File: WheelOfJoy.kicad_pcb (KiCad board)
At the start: 2 copper layers, 89.2 x 87.9 mm, 39 parts, among them CN1 JOY1, CN2 JOY2, CN3 JOY3, CN4 JOY4, CN5 JOY5, CN6 JOY6, CN7 JOY7, CN8 JOY8, CN9 DB15F, U1 CD4051B, U2 CD4051B, U3 CD4051B, U4 CD4051B, U5 CD4051B

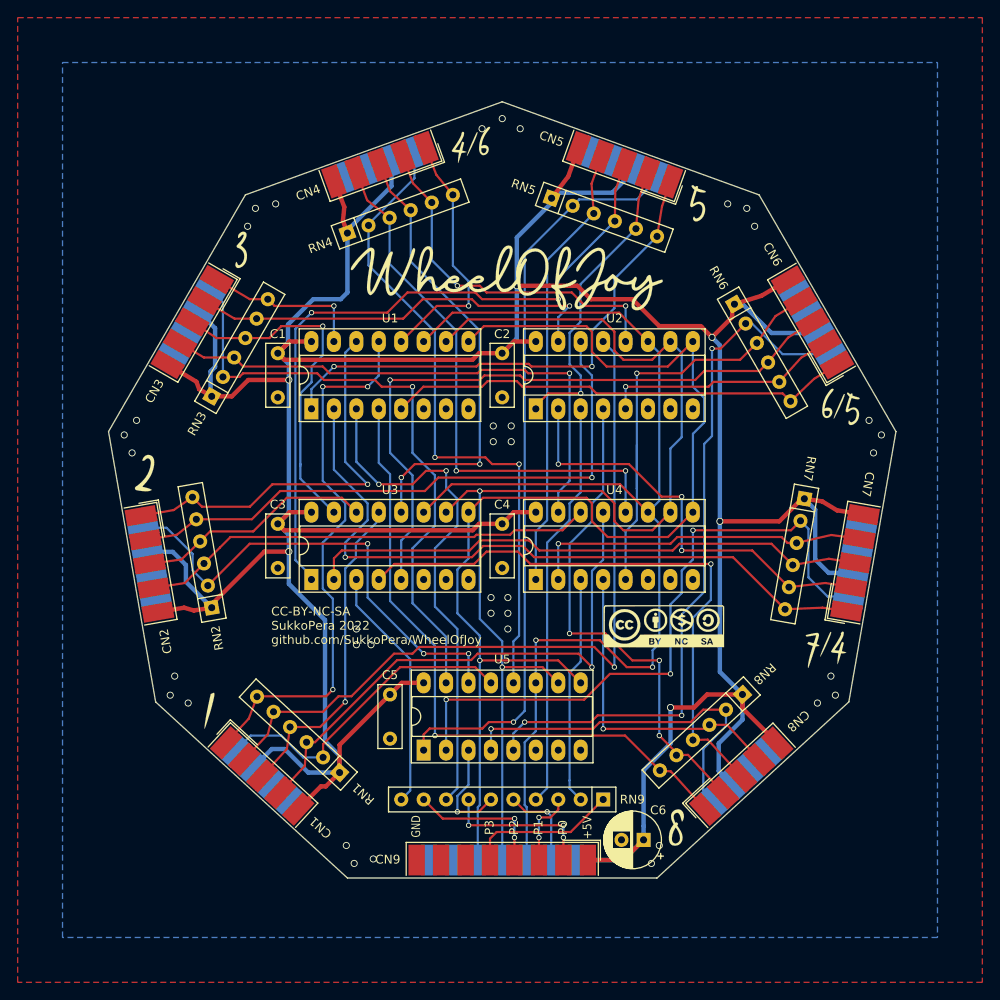
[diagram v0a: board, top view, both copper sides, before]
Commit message: WIP
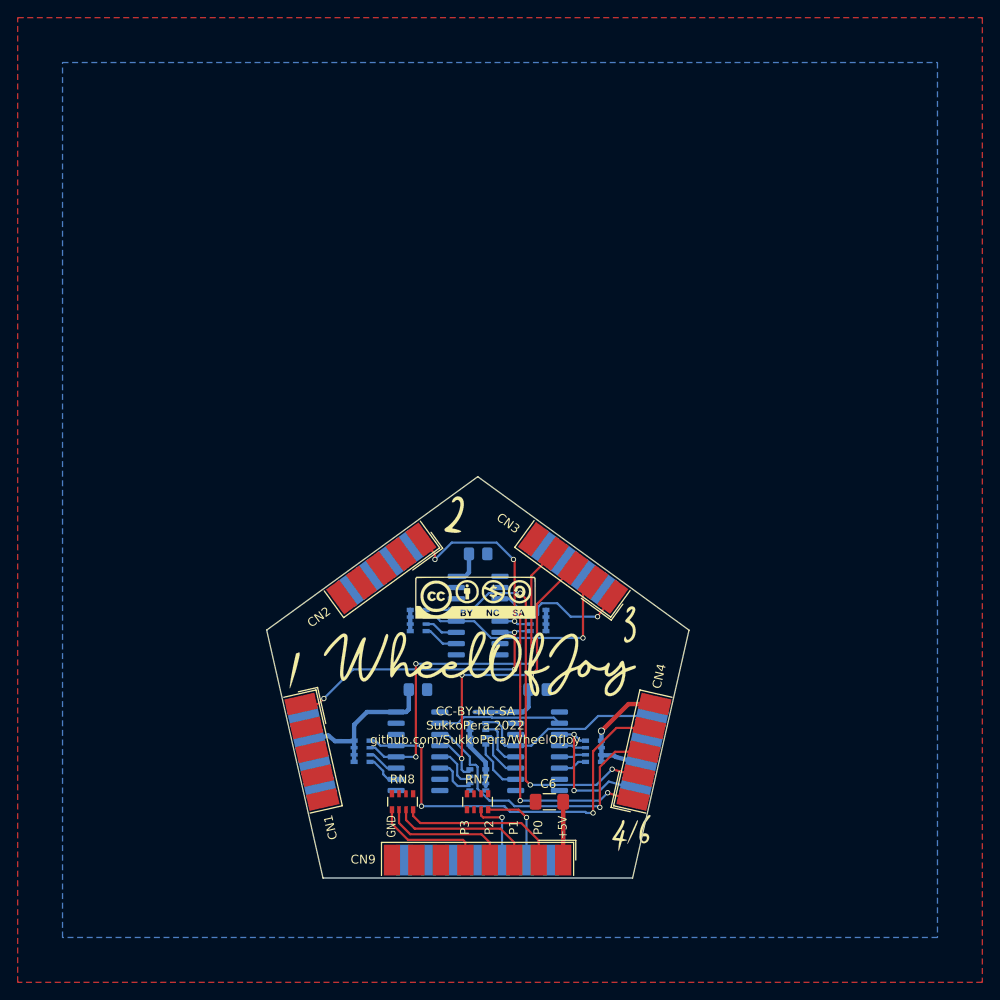
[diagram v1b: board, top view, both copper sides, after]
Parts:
- removed C4, C5: 100n, Capacitor_THT:C_Disc_D7.0mm_W2.5mm_P5.00mm
- removed CN5: JOY5, Connector_Dsub:DSUB-9_Male_EdgeMount_P2.77mm
- removed CN6: JOY6, Connector_Dsub:DSUB-9_Male_EdgeMount_P2.77mm
- removed CN7: JOY7, Connector_Dsub:DSUB-9_Male_EdgeMount_P2.77mm
- removed CN8: JOY8, Connector_Dsub:DSUB-9_Male_EdgeMount_P2.77mm
- removed RN9: 100, Resistor_THT:R_Array_SIP10
- removed U4, U5: CD4051B, Package_DIP:DIP-16_W7.62mm_Socket_LongPads
- removed V6: PORT5_NO, WheelOfJoy:port5
- removed V7: PORT6_NO, WheelOfJoy:port6
- removed V8: PORT7_NO, WheelOfJoy:port7
- removed V9: PORT8_NO, WheelOfJoy:port8
- C1, C2, C3: footprint Capacitor_THT:C_Disc_D7.0mm_W2.5mm_P5.00mm -> Capacitor_SMD:C_0805_2012Metric_Pad1.18x1.45mm_HandSolder; moved to B.Cu
- C6: footprint Capacitor_THT:CP_Radial_D6.3mm_P2.50mm -> Capacitor_SMD:C_1206_3216Metric_Pad1.33x1.80mm_HandSolder
- RN1, RN2, RN3, RN4, RN5, RN6: footprint Resistor_THT:R_Array_SIP6 -> Resistor_SMD:R_Array_Convex_4x0603; moved to B.Cu
- RN7, RN8: value 4.7k -> 100; footprint Resistor_THT:R_Array_SIP6 -> Resistor_SMD:R_Array_Convex_4x0603
- U1, U2, U3: value CD4051B -> 74LS153; footprint Package_DIP:DIP-16_W7.62mm_Socket_LongPads -> Package_SO:SOIC-16_3.9x9.9mm_P1.27mm; moved to B.Cu
- moved V5 80.0 mm to (166.0, 130.4)
- moved CN4 72.9 mm to (167.4, 121.2), turned to 77.2 degrees
- moved RN4 63.6 mm to (148.6, 124.4), turned to 180 degrees
- moved RN5 61.2 mm to (148.6, 119.2), turned to 180 degrees
- moved V4 61.1 mm to (166.8, 106.8)
- moved RN6 53.1 mm to (161.7, 121.2), turned to 180 degrees
- moved CN3 51.3 mm to (159.4, 100.4), turned to 144 degrees
- moved RN7 50.5 mm to (148.6, 126.9), turned to 90 degrees
- moved V0 43.8 mm to (148.8, 111.3)
- moved RN3 43.6 mm to (135.5, 121.2), turned to 180 degrees
- moved U2 41.0 mm to (141.8, 121.2), turned to 180 degrees
- moved RN8 40.4 mm to (140.1, 126.9), turned to 90 degrees
- moved C2 39.3 mm to (141.8, 114.2), turned to 0 degrees
- moved RN2 37.0 mm to (155.4, 106.4), turned to 180 degrees
- moved V3 35.4 mm to (146.4, 94.4)
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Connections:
- CN1 pad 9: (no net) -> Net-(CN1-Pad9)
- CN2 pad 9: (no net) -> Net-(CN2-Pad9)
- CN3 pad 9: (no net) -> Net-(CN3-Pad9)
- CN4 pad 9: (no net) -> Net-(CN4-Pad9)
- CN9 pad 11: /d5 -> Net-(CN9-Pad11)
- CN9 pad 14: (no net) -> Net-(CN9-Pad14)
- CN9 pad 6: (no net) -> /~reset
- CN9 pad 7: (no net) -> Net-(CN9-Pad7)
- RN1 pad 1: +5V -> Net-(CN4-Pad2)
- RN1 pad 2: Net-(CN1-Pad6) -> Net-(CN3-Pad2)
- RN1 pad 3: Net-(CN1-Pad4) -> Net-(CN2-Pad2)
- RN1 pad 4: Net-(CN1-Pad3) -> Net-(CN1-Pad2)
- RN1 pad 5: Net-(CN1-Pad2) -> +5V
- RN1 pad 6: Net-(CN1-Pad1) -> +5V
- RN2 pad 2: Net-(CN2-Pad6) -> +5V
- RN2 pad 3: Net-(CN2-Pad4) -> +5V
- RN2 pad 4: Net-(CN2-Pad3) -> +5V
- RN2 pad 5: Net-(CN2-Pad2) -> Net-(CN1-Pad1)
- RN3 pad 1: +5V -> Net-(CN4-Pad4)
- RN3 pad 2: Net-(CN3-Pad6) -> Net-(CN3-Pad4)
- RN3 pad 3: Net-(CN3-Pad4) -> Net-(CN2-Pad4)
- RN3 pad 4: Net-(CN3-Pad3) -> Net-(CN1-Pad4)
- RN3 pad 5: Net-(CN3-Pad2) -> +5V
- RN3 pad 6: Net-(CN3-Pad1) -> +5V
- RN4 pad 2: Net-(CN4-Pad6) -> +5V
- RN4 pad 3: Net-(CN4-Pad4) -> +5V
- RN4 pad 4: Net-(CN4-Pad3) -> +5V
- RN4 pad 5: Net-(CN4-Pad2) -> Net-(CN1-Pad3)
- RN4 pad 6: Net-(CN4-Pad1) -> Net-(CN2-Pad3)
- RN5 pad 1: +5V -> Net-(CN4-Pad9)
- RN5 pad 2: Net-(CN5-Pad6) -> Net-(CN3-Pad9)
- RN5 pad 3: Net-(CN5-Pad4) -> Net-(CN2-Pad9)
- RN5 pad 4: Net-(CN5-Pad3) -> Net-(CN1-Pad9)
- RN5 pad 5: Net-(CN5-Pad2) -> +5V
- RN5 pad 6: Net-(CN5-Pad1) -> +5V
- RN6 pad 2: Net-(CN6-Pad6) -> +5V
- RN6 pad 3: Net-(CN6-Pad4) -> +5V
- RN6 pad 4: Net-(CN6-Pad3) -> +5V
- RN6 pad 5: Net-(CN6-Pad2) -> Net-(CN1-Pad6)
- RN6 pad 6: Net-(CN6-Pad1) -> Net-(CN2-Pad6)
- RN7 pad 1: +5V -> Net-(RN7-Pad1)
- RN7 pad 3: Net-(CN7-Pad4) -> Net-(CN9-Pad11)
- RN7 pad 4: Net-(CN7-Pad3) -> Net-(CN9-Pad10)
- RN7 pad 5: Net-(CN7-Pad2) -> /d4
- RN7 pad 6: Net-(CN7-Pad1) -> /d5
- RN8 pad 1: +5V -> Net-(CN9-Pad5)
- RN8 pad 2: Net-(CN8-Pad6) -> Net-(CN9-Pad4)
- RN8 pad 3: Net-(CN8-Pad4) -> Net-(CN9-Pad3)
- RN8 pad 4: Net-(CN8-Pad3) -> Net-(CN9-Pad2)
- RN8 pad 5: Net-(CN8-Pad2) -> /d0
- RN8 pad 6: Net-(CN8-Pad1) -> /d1
- U1 pad 1: Net-(CN5-Pad1) -> GND
- U1 pad 10: /d6 -> Net-(CN1-Pad2)
- U1 pad 11: /d5 -> Net-(CN2-Pad2)
- U1 pad 12: Net-(CN4-Pad1) -> Net-(CN3-Pad2)
- U1 pad 13: Net-(CN1-Pad1) -> Net-(CN4-Pad2)
- U1 pad 14: Net-(CN2-Pad1) -> /d6
- U1 pad 15: Net-(CN3-Pad1) -> GND
- U1 pad 2: Net-(CN7-Pad1) -> /d7
- U1 pad 3: /d0 -> Net-(CN4-Pad1)
- U1 pad 4: Net-(CN8-Pad1) -> Net-(CN3-Pad1)
- U1 pad 5: Net-(CN6-Pad1) -> Net-(CN2-Pad1)
- U1 pad 6: GND -> Net-(CN1-Pad1)
- U1 pad 7: GND -> /d0
- U1 pad 9: /d7 -> /d1
- U2 pad 1: Net-(CN5-Pad2) -> GND
- U2 pad 10: /d6 -> Net-(CN1-Pad4)
- U2 pad 11: /d5 -> Net-(CN2-Pad4)
- U2 pad 12: Net-(CN4-Pad2) -> Net-(CN3-Pad4)
- U2 pad 13: Net-(CN1-Pad2) -> Net-(CN4-Pad4)
- U2 pad 14: Net-(CN2-Pad2) -> /d6
- U2 pad 15: Net-(CN3-Pad2) -> GND
- U2 pad 2: Net-(CN7-Pad2) -> /d7
- U2 pad 3: /d1 -> Net-(CN4-Pad3)
- U2 pad 4: Net-(CN8-Pad2) -> Net-(CN3-Pad3)
- U2 pad 5: Net-(CN6-Pad2) -> Net-(CN2-Pad3)
- U2 pad 6: GND -> Net-(CN1-Pad3)
- U2 pad 7: GND -> /d2
- U2 pad 9: /d7 -> /d3
- U3 pad 1: Net-(CN5-Pad3) -> GND
- U3 pad 10: /d6 -> Net-(CN1-Pad9)
- U3 pad 11: /d5 -> Net-(CN2-Pad9)
- U3 pad 12: Net-(CN4-Pad3) -> Net-(CN3-Pad9)
- U3 pad 13: Net-(CN1-Pad3) -> Net-(CN4-Pad9)
- U3 pad 14: Net-(CN2-Pad3) -> /d6
- U3 pad 15: Net-(CN3-Pad3) -> GND
- U3 pad 2: Net-(CN7-Pad3) -> /d7
- U3 pad 3: /d2 -> Net-(CN4-Pad6)
- U3 pad 4: Net-(CN8-Pad3) -> Net-(CN3-Pad6)
- U3 pad 5: Net-(CN6-Pad3) -> Net-(CN2-Pad6)
- U3 pad 6: GND -> Net-(CN1-Pad6)
- U3 pad 7: GND -> /d4
- U3 pad 9: /d7 -> /d5
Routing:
- net +5V: track 461.8 -> 66.4 mm, vias 6 -> 1
- net /d5: track 134.9 -> 0.00 mm, vias 2 -> 0
- net /d6: track 131.0 -> 0.00 mm, vias 2 -> 0
- net /d7: track 134.7 -> 14.2 mm, vias 1 -> 0
- net Net-(CN5-Pad6): track 84.9 -> 0.00 mm, vias 1 -> 0
- net Net-(CN1-Pad2): track 86.5 -> 3.99 mm, vias 1 -> 0
- net Net-(CN6-Pad6): track 81.6 -> 0.00 mm, vias 3 -> 0
- net Net-(CN7-Pad1): track 79.7 -> 0.00 mm, vias 1 -> 0
- net Net-(CN5-Pad3): track 79.0 -> 0.00 mm, vias 2 -> 0
- net Net-(CN6-Pad3): track 75.1 -> 0.00 mm, vias 1 -> 0
- net Net-(RN7-Pad2): track 74.6 -> 0.00 mm, vias 3 -> 0
- net Net-(CN8-Pad1): track 73.8 -> 0.00 mm, vias 1 -> 0
- net Net-(CN8-Pad3): track 67.6 -> 0.00 mm, vias 1 -> 0
- net Net-(CN3-Pad6): track 70.0 -> 3.05 mm, vias 1 -> 0
- net Net-(CN2-Pad2): track 69.1 -> 3.80 mm, vias 1 -> 0
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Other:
- board size 89.2 x 87.9 mm -> 47.8 x 45.4 mm
